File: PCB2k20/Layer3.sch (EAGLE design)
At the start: 45 parts

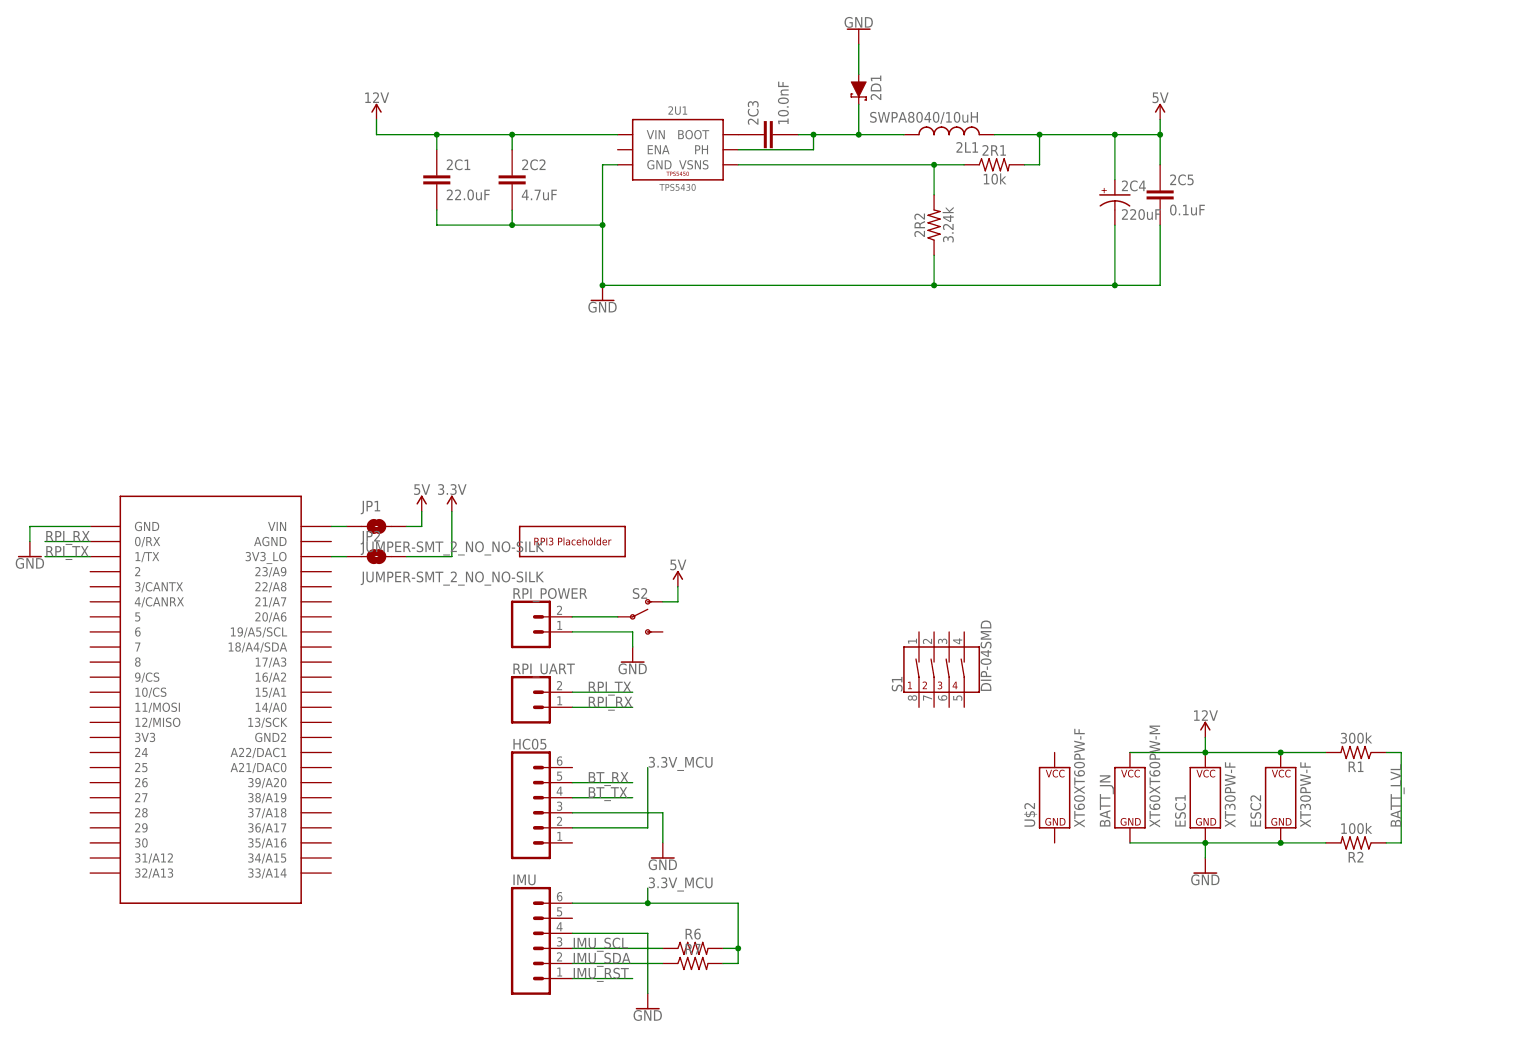
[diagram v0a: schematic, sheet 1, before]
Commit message: done just need to silkscreen now!!!
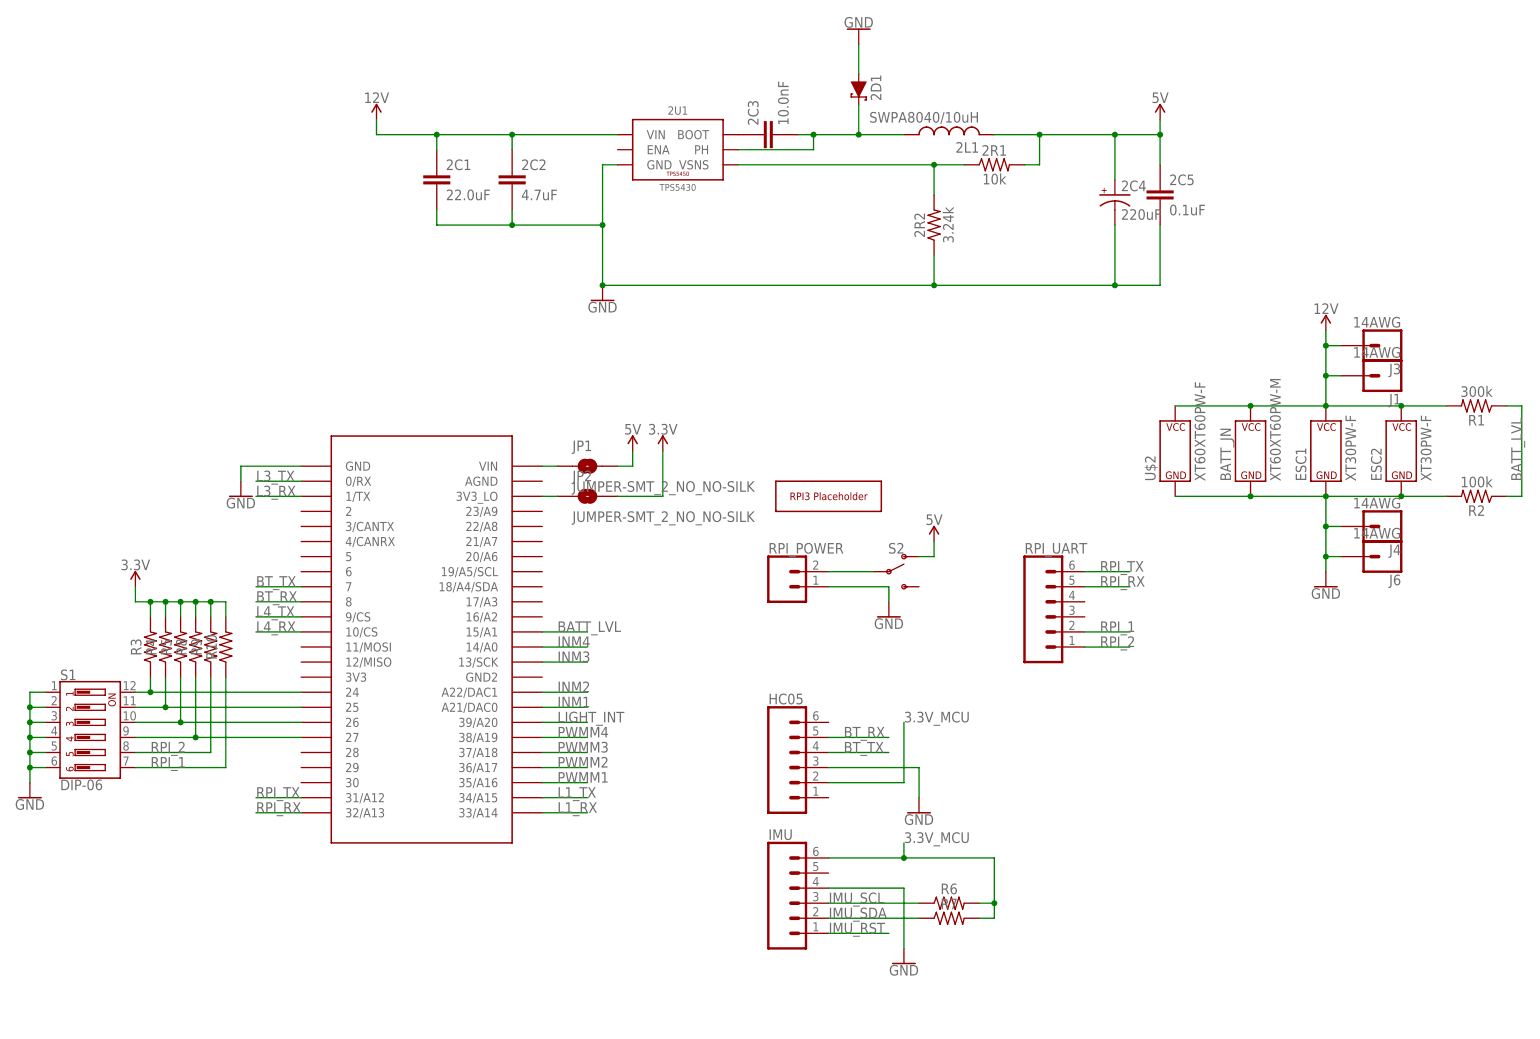
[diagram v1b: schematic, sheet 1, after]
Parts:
- added J1, J3, J4, J6: 14AWG, JH:14AWG
- added J2: CONN_03, JH:CONN_03
- added R10, R3, R4, R5, R8, R9: (no value), JH:RESISTOR0603
- added X1: BM10B-SRSS-TB, con-JST SH:BM10B-SRSS-TB
- RPI_UART: device SparkFun-Connectors:CONN_02LOCK -> SparkFun-Connectors:CONN_06LOCK
- S1: value DIP-04SMD -> DIP-06; device SparkFun-Switches:DIP-04SMD -> SparkFun-Switches:DIP-06
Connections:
- new net INM1: U$1.A21/DAC0, X1.8
- new net INM2: U$1.A22/DAC1, X1.6
- new net INM3: U$1.13/SCK, X1.4
- new net INM4: U$1.14/A0, X1.2
- new net L1_RX: U$1.33/A14, X1.9
- new net L1_TX: U$1.34/A15, X1.10
- new net LIGHT_INT: J2.1, U$1.39/A20
- new net N$10: R3.1, S1.12, U$1.24
- new net N$11: R5.1, S1.10, U$1.26
- new net N$12: R8.1, S1.9, U$1.27
- new net N$5: R4.1, S1.11, U$1.25
- new net PWMM1: U$1.35/A16, X1.7
- new net PWMM2: U$1.36/A17, X1.5
- new net PWMM3: U$1.37/A18, X1.3
- new net PWMM4: U$1.38/A19, X1.1
- new net RPI_1: R10.1, RPI_UART.2, S1.7
- new net RPI_2: R9.1, RPI_UART.1, S1.8
- net 12V: now also J1.1, J3.1, U$2.P$V+
- net 3.3V: now also J2.3, R10.2, R3.2, R4.2, R5.2, R8.2, R9.2
- net BATT_LVL: now also U$1.15/A1
- net BT_RX: now also U$1.8
- net BT_TX: now also U$1.7
- net GND: now also J2.2, J4.1, J6.1, S1.1, S1.2, S1.3, S1.4, S1.5, S1.6, U$2.P$V-
- net L3_RX: now also U$1.1/TX
- net L3_TX: now also U$1.0/RX
- net L4_RX: now also U$1.10/CS
- net L4_TX: now also U$1.9/CS
- net RPI_RX: now also RPI_UART.5, U$1.32/A13; no longer RPI_UART.1, U$1.0/RX
- net RPI_TX: now also RPI_UART.6, U$1.31/A12; no longer RPI_UART.2, U$1.1/TX
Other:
- moved on the sheet: BATT_JN, ESC1, ESC2, HC05, IMU, JP1, JP2, R1, R2, R6, R7, RPI_POWER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
